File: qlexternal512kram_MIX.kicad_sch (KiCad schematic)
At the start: 15 parts, among them J1 QL_SLOT_DIN41612_CARD, J2 QL_SLOT_DIN41612_CARD, U1 HM628512BLFP-7, U2 GAL16V8B-25QP, U3 LM1117-5.0

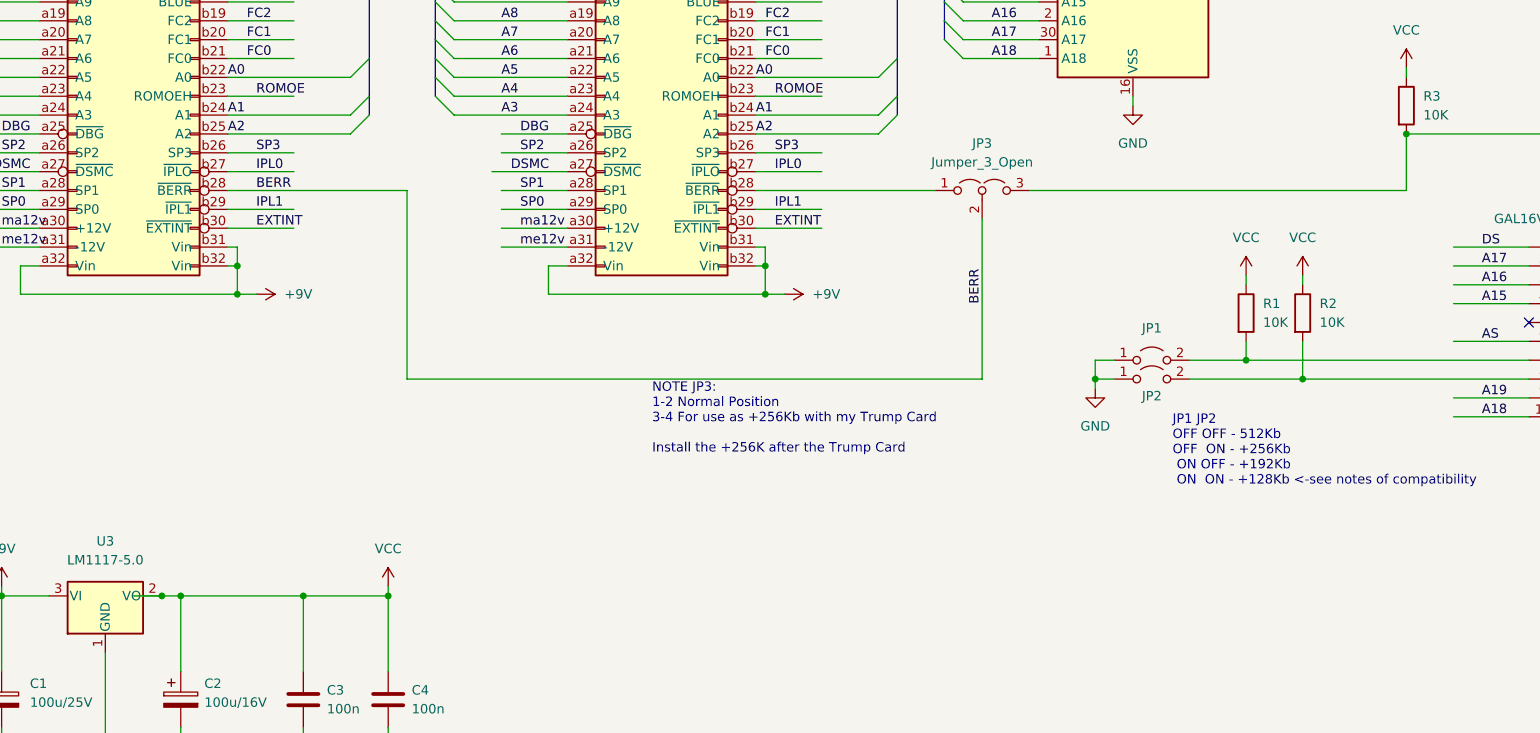
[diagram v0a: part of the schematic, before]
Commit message: version pre-release 1
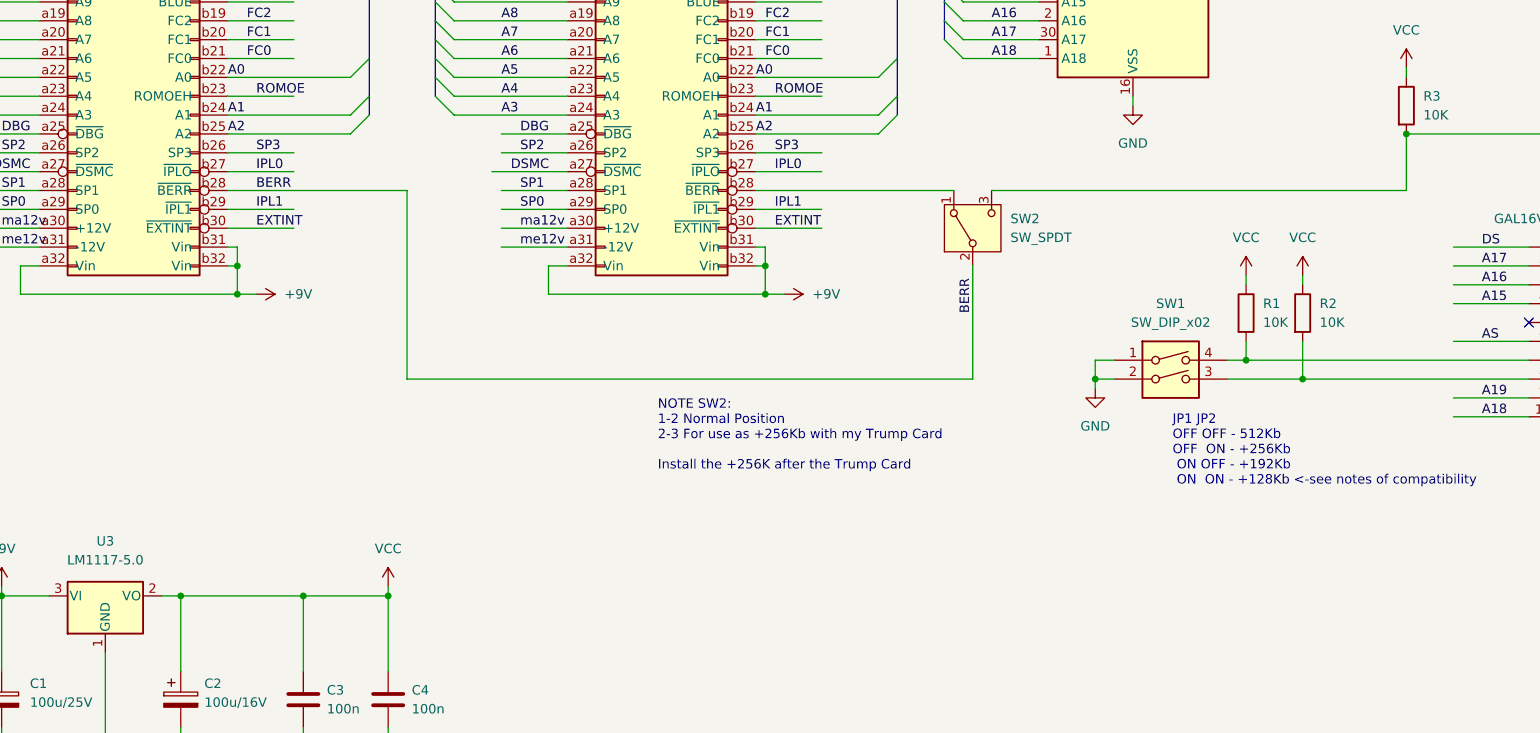
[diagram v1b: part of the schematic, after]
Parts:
- removed JP1, JP2: Jumper_2_Open, Jumper:SolderJumper-2_P1.3mm_Open_Pad1.0x1.5mm, symbol Jumper:Jumper_2_Open
- removed JP3: Jumper_3_Open, Jumper:SolderJumper-3_P1.3mm_Open_Pad1.0x1.5mm, symbol Jumper:Jumper_3_Open
- added SW1: SW_DIP_x02, Button_Switch_SMD:SW_DIP_SPSTx02_Slide_KingTek_DSHP02TS_W7.62mm_P1.27mm, symbol Switch:SW_DIP_x02
- added SW2: SW_SPDT, Button_Switch_SMD:SW_SPDT_PCM12, symbol Switch:SW_SPDT
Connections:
- net BERR: now also SW2.2 (B)
- net GND: now also SW1.1, SW1.2
- net at J2.b28 (~{BERR}): now also SW2.1 (A)
- net at R3.2, U2.17 (I03): now also SW2.3 (C)
- net at R1.2, U2.7 (I7): now also SW1.4
- net at R2.2, U2.8 (I8): now also SW1.3
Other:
- note added: "NOTE SW2: 1-2 Normal Position 2-3 For use as +256Kb with my Trump Card Install the +256K after the Trump Card"
- note removed: "NOTE JP3: 1-2 Normal Position 3-4 For use as +256Kb with my Trump Card Install the +256K after the Trump Card"
